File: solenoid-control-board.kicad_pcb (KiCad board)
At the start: 2 copper layers, 72 x 48 mm, 39 parts, among them J1 505578-0671, J2 505578-0671, J3 SM04B-GHS-TB, J4 XT30PW-M30.G.Y1, J5 XT30PW-M30.G.Y1, M1 CSD16323Q3, M2 CSD16323Q3, M3 CSD16323Q3, M4 CSD16323Q3, M5 CSD16323Q3, M6 CSD16323Q3, U7 PCA9534PWR

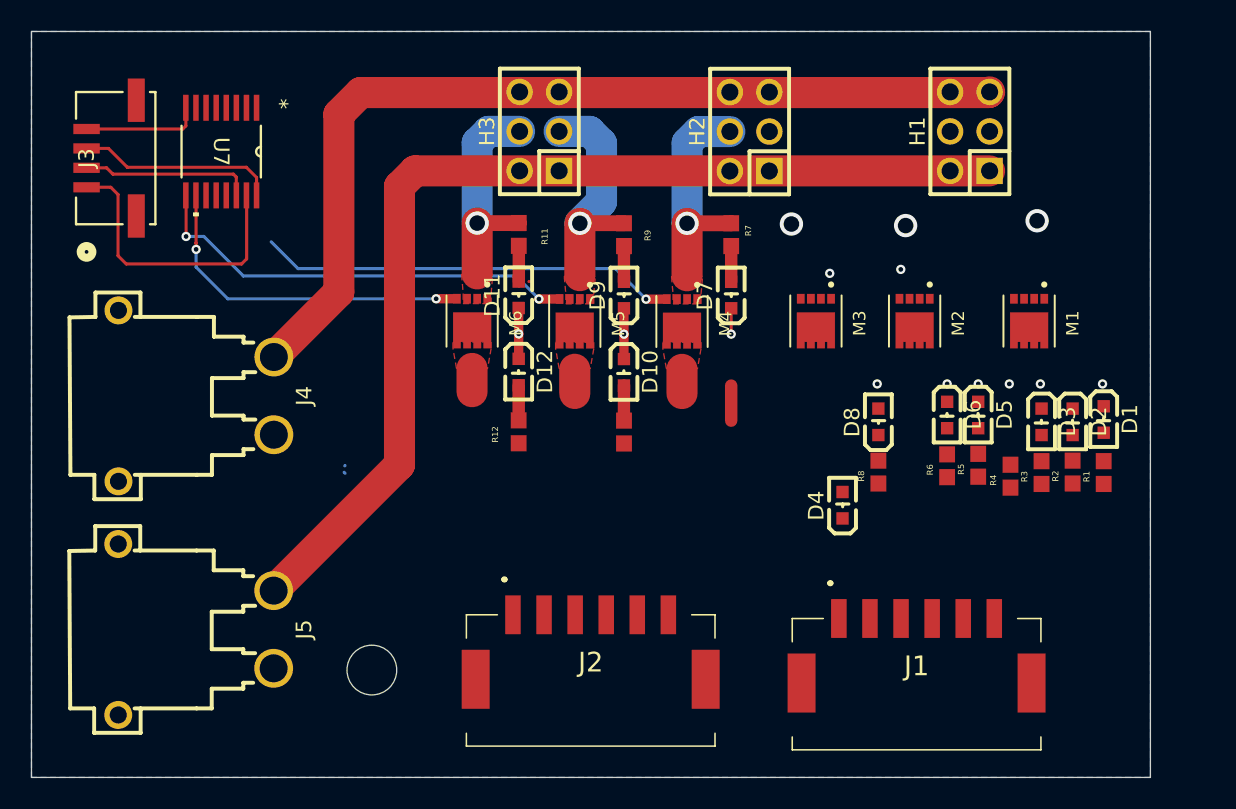
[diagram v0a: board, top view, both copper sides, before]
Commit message: Finished almost everything
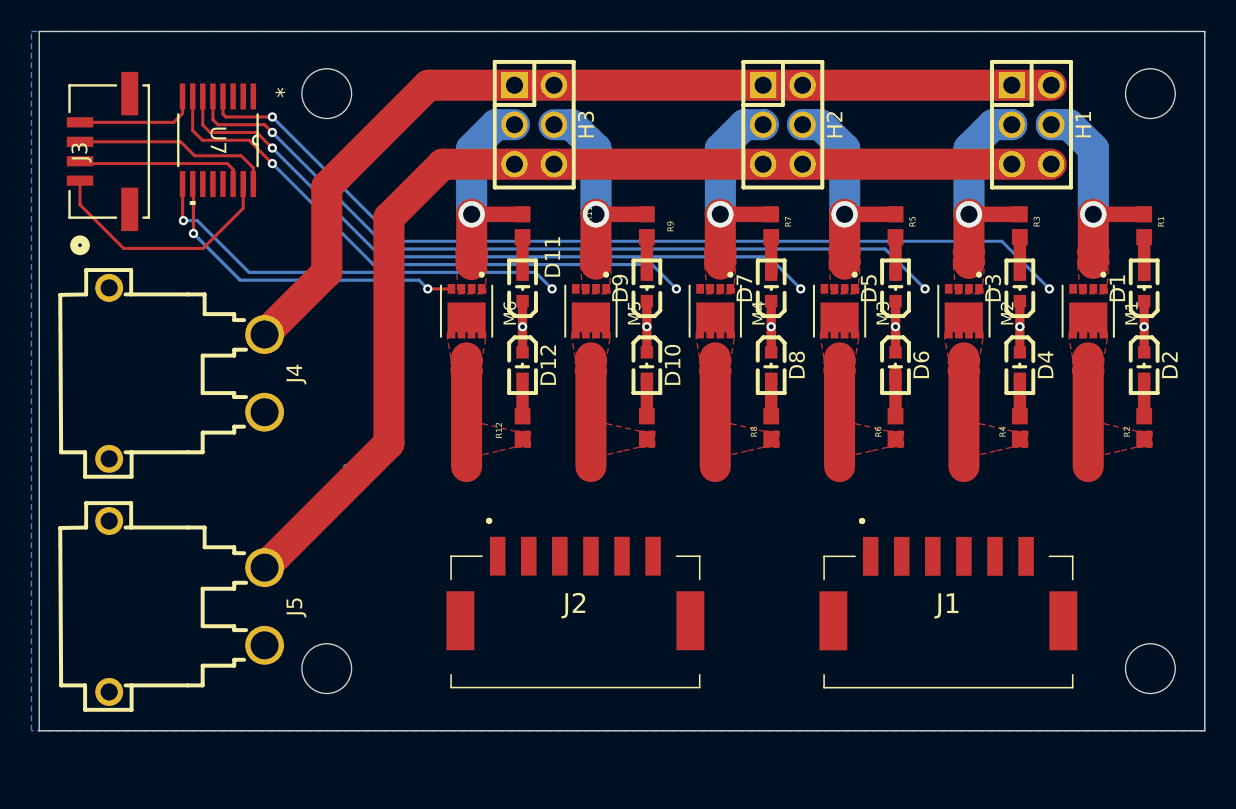
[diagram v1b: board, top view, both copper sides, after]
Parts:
- moved R5 16.3 mm to (146.6, 64.5), turned to -90 degrees
- moved R1 16.1 mm to (162.6, 64.5), turned to -90 degrees
- moved R3 15.9 mm to (154.6, 64.5), turned to -90 degrees
- moved D4 14.5 mm to (154.6, 73.5), turned to -90 degrees
- moved D5 9.76 mm to (146.6, 68.5), turned to 90 degrees
- moved D1 8.86 mm to (162.6, 68.5), turned to 90 degrees
- moved D3 8.73 mm to (154.6, 68.5), turned to 90 degrees
- moved D8 7.79 mm to (138.6, 73.5), turned to -90 degrees
- moved R8 7.46 mm to (138.6, 77.5)
- moved D2 5.86 mm to (162.6, 73.5)
- moved R2 5.42 mm to (162.6, 77.5)
- moved D6 4.60 mm to (146.6, 73.5)
- moved J1 4.49 mm to (150.0, 90.0)
- moved R6 4.12 mm to (146.6, 77.5)
- moved H1 3.99 mm to (155.3, 58.0), turned to -90 degrees
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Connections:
- H1 pad 1: +6V -> +12V
- H1 pad 2: +6V -> +12V
- H1 pad 3: SRC_1 -> SRC_2
- H1 pad 4: SRC_2 -> SRC_1
- H1 pad 5: +12V -> +6V
- H1 pad 6: +12V -> +6V
- H2 pad 1: +6V -> +12V
- H2 pad 2: +6V -> +12V
- H2 pad 3: SRC_3 -> SRC_4
- H2 pad 4: SRC_4 -> SRC_3
- H2 pad 5: +12V -> +6V
- H2 pad 6: +12V -> +6V
- H3 pad 1: +6V -> +12V
- H3 pad 2: +6V -> +12V
- H3 pad 3: SRC_5 -> SRC_6
- H3 pad 4: SRC_6 -> SRC_5
- H3 pad 5: +12V -> +6V
- H3 pad 6: +12V -> +6V
- J1 pad 1: SOL_3_PWR -> GND
- J1 pad 2: GND -> SOL_3_PWR
- J1 pad 3: SOL_2_PWR -> GND
- J1 pad 4: GND -> SOL_2_PWR
- J1 pad 5: SOL_1_PWR -> GND
- J1 pad 6: GND -> SOL_1_PWR
- J2 pad 1: SOL_6_PWR -> GND
- J2 pad 2: GND -> SOL_6_PWR
- J2 pad 3: SOL_5_PWR -> GND
- J2 pad 4: GND -> SOL_5_PWR
- J2 pad 5: SOL_4_PWR -> GND
- J2 pad 6: GND -> SOL_4_PWR
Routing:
- net GATE_1: track 0.00 -> 59.0 mm, vias 0 -> 2
- net GATE_2: track 0.00 -> 51.8 mm, vias 0 -> 2
- net GATE_3: track 0.00 -> 44.7 mm, vias 0 -> 2
- net SRC_3: track 0.00 -> 14.1 mm
- net SRC_2: track 0.00 -> 14.1 mm
- net SRC_1: track 0.00 -> 14.0 mm
- net GATE_4: track 26.7 -> 37.5 mm, vias 1 -> 2
- net GND: track 11.4 -> 20.3 mm, vias 9 -> 6
- net SOL_5_PWR: track 0.00 -> 7.00 mm
- net SOL_4_PWR: track 0.00 -> 7.00 mm
- net SOL_3_PWR: track 0.00 -> 7.00 mm
- net SOL_2_PWR: track 0.00 -> 7.00 mm
- net SOL_1_PWR: track 0.00 -> 7.00 mm
- net SOL_6_PWR: track 1.50 -> 7.00 mm
- net Net-(D6-Pad1): track 0.00 -> 2.91 mm
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- added copper zone on F.Cu, net SOL_1_PWR
- added copper zone on F.Cu, net SOL_2_PWR
- added copper zone on F.Cu, net SOL_3_PWR
- added copper zone on F.Cu, net SOL_4_PWR
- added copper zone on F.Cu, net SOL_5_PWR
- added copper zone on F.Cu, net SRC_1
- added copper zone on F.Cu, net SRC_2
- added copper zone on F.Cu, net SRC_3
- added copper zone on F.Cu, net SRC_4
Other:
- board size 72 x 48 mm -> 75 x 45 mm
